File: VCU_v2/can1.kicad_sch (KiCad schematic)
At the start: 6 parts, among them U10 MCP2562FD-E/SN

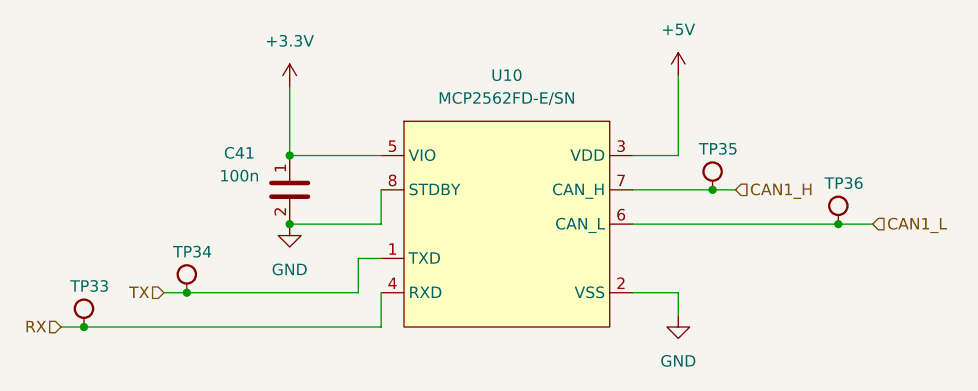
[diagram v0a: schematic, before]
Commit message: placements friggin 80% friggin done shoutout epstein
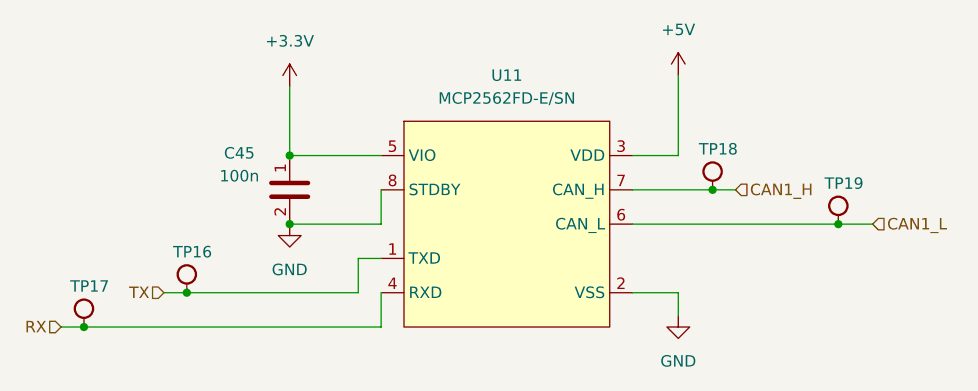
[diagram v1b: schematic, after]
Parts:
- renumbered C41 to C45, TP34 to TP16, TP33 to TP17, TP35 to TP18, TP36 to TP19, U10 to U11
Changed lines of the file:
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@@
 		(dnp no)
 		(fields_autoplaced yes)
-		(property "Reference" "#PWR055"
+		(property "Reference" "#PWR075"
 			(at 114.3 66.04 0)
 			(effects
@@
 			(project ""
 				(path "/4ee6c2ad-9a1b-4276-b3cf-1cc8dc52967e/9e80ce31-2e03-4996-9ce1-7444f7c213d1/6a8587bb-cd3f-4184-88f1-dc60fd50b84f"
-					(reference "#PWR055")
+					(reference "#PWR075")
 					(unit 1)
 				)
@@
 		(on_board yes)
 		(dnp no)
-		(property "Reference" "TP36"
+		(property "Reference" "TP19"
 			(at 173.7368 72.2137 0)
 			(effects
@@
 			(project "VCU_v1"
 				(path "/4ee6c2ad-9a1b-4276-b3cf-1cc8dc52967e/9e80ce31-2e03-4996-9ce1-7444f7c213d1/6a8587bb-cd3f-4184-88f1-dc60fd50b84f"
-					(reference "TP36")
+					(reference "TP19")
 					(unit 1)
 				)
@@
 		(dnp no)
 		(fields_autoplaced yes)
-		(property "Reference" "#PWR057"
+		(property "Reference" "#PWR076"
 			(at 157.48 64.77 0)
 			(effects
@@
 			(project ""
 				(path "/4ee6c2ad-9a1b-4276-b3cf-1cc8dc52967e/9e80ce31-2e03-4996-9ce1-7444f7c213d1/6a8587bb-cd3f-4184-88f1-dc60fd50b84f"
-					(reference "#PWR057")
+					(reference "#PWR076")
 					(unit 1)
 				)
@@
 		(on_board yes)
 		(dnp no)
-		(property "Reference" "TP34"
+		(property "Reference" "TP16"
 			(at 101.3468 79.8337 0)
 			(effects
@@
 			(project "VCU_v1"
 				(path "/4ee6c2ad-9a1b-4276-b3cf-1cc8dc52967e/9e80ce31-2e03-4996-9ce1-7444f7c213d1/6a8587bb-cd3f-4184-88f1-dc60fd50b84f"
-					(reference "TP34")
+					(reference "TP16")
 					(unit 1)
 				)
@@
 		(on_board yes)
 		(dnp no)
-		(property "Reference" "TP35"
+		(property "Reference" "TP18"
 			(at 159.7668 68.4037 0)
 			(effects
@@
 			(project "VCU_v1"
 				(path "/4ee6c2ad-9a1b-4276-b3cf-1cc8dc52967e/9e80ce31-2e03-4996-9ce1-7444f7c213d1/6a8587bb-cd3f-4184-88f1-dc60fd50b84f"
-					(reference "TP35")
+					(reference "TP18")
 					(unit 1)
 				)
@@
 		(on_board yes)
 		(dnp no)
-		(property "Reference" "TP33"
+		(property "Reference" "TP17"
 			(at 89.9168 83.6437 0)
 			(effects
@@
 			(project "VCU_v1"
 				(path "/4ee6c2ad-9a1b-4276-b3cf-1cc8dc52967e/9e80ce31-2e03-4996-9ce1-7444f7c213d1/6a8587bb-cd3f-4184-88f1-dc60fd50b84f"
-					(reference "TP33")
+					(reference "TP17")
 					(unit 1)
 				)
@@
 		(on_board yes)
 		(dnp no)
-		(property "Reference" "U10"
+		(property "Reference" "U11"
 			(at 138.43 60.96 0)
 			(effects
@@
 			(project ""
 				(path "/4ee6c2ad-9a1b-4276-b3cf-1cc8dc52967e/9e80ce31-2e03-4996-9ce1-7444f7c213d1/6a8587bb-cd3f-4184-88f1-dc60fd50b84f"
-					(reference "U10")
+					(reference "U11")
 					(unit 1)
 				)
@@
 		(dnp no)
 		(fields_autoplaced yes)
-		(property "Reference" "#PWR058"
+		(property "Reference" "#PWR077"
 			(at 157.48 93.98 0)
 			(effects
@@
 			(project ""
 				(path "/4ee6c2ad-9a1b-4276-b3cf-1cc8dc52967e/9e80ce31-2e03-4996-9ce1-7444f7c213d1/6a8587bb-cd3f-4184-88f1-dc60fd50b84f"
-					(reference "#PWR058")
+					(reference "#PWR077")
 					(unit 1)
 				)
@@
 		(on_board yes)
 		(dnp no)
-		(property "Reference" "C41"
+		(property "Reference" "C45"
 			(at 108.712 69.596 0)
 			(effects
@@
 			(project ""
 				(path "/4ee6c2ad-9a1b-4276-b3cf-1cc8dc52967e/9e80ce31-2e03-4996-9ce1-7444f7c213d1/6a8587bb-cd3f-4184-88f1-dc60fd50b84f"
-					(reference "C41")
+					(reference "C45")
 					(unit 1)
 				)
@@
 		(dnp no)
 		(fields_autoplaced yes)
-		(property "Reference" "#PWR056"
+		(property "Reference" "#PWR012"
 			(at 114.3 83.82 0)
 			(effects
@@
 			(project ""
 				(path "/4ee6c2ad-9a1b-4276-b3cf-1cc8dc52967e/9e80ce31-2e03-4996-9ce1-7444f7c213d1/6a8587bb-cd3f-4184-88f1-dc60fd50b84f"
-					(reference "#PWR056")
+					(reference "#PWR012")
 					(unit 1)
 				)

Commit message: vcu v2 schematics done
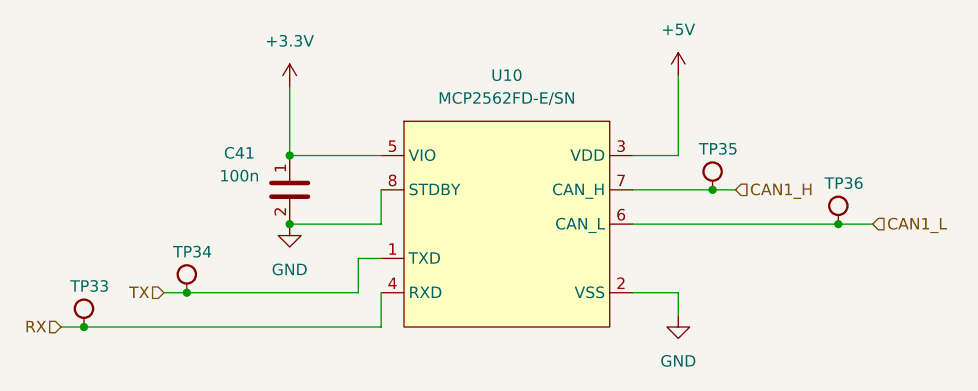
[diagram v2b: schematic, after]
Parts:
- renumbered C45 to C41, TP17 to TP33, TP16 to TP34, TP18 to TP35, TP19 to TP36, U11 to U10
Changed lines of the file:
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@@
 		(dnp no)
 		(fields_autoplaced yes)
-		(property "Reference" "#PWR075"
+		(property "Reference" "#PWR055"
 			(at 114.3 66.04 0)
 			(effects
@@
 			(project ""
 				(path "/4ee6c2ad-9a1b-4276-b3cf-1cc8dc52967e/9e80ce31-2e03-4996-9ce1-7444f7c213d1/6a8587bb-cd3f-4184-88f1-dc60fd50b84f"
-					(reference "#PWR075")
+					(reference "#PWR055")
 					(unit 1)
 				)
@@
 		(on_board yes)
 		(dnp no)
-		(property "Reference" "TP19"
+		(property "Reference" "TP36"
 			(at 173.7368 72.2137 0)
 			(effects
@@
 			(project "VCU_v1"
 				(path "/4ee6c2ad-9a1b-4276-b3cf-1cc8dc52967e/9e80ce31-2e03-4996-9ce1-7444f7c213d1/6a8587bb-cd3f-4184-88f1-dc60fd50b84f"
-					(reference "TP19")
+					(reference "TP36")
 					(unit 1)
 				)
@@
 		(dnp no)
 		(fields_autoplaced yes)
-		(property "Reference" "#PWR076"
+		(property "Reference" "#PWR057"
 			(at 157.48 64.77 0)
 			(effects
@@
 			(project ""
 				(path "/4ee6c2ad-9a1b-4276-b3cf-1cc8dc52967e/9e80ce31-2e03-4996-9ce1-7444f7c213d1/6a8587bb-cd3f-4184-88f1-dc60fd50b84f"
-					(reference "#PWR076")
+					(reference "#PWR057")
 					(unit 1)
 				)
@@
 		(on_board yes)
 		(dnp no)
-		(property "Reference" "TP16"
+		(property "Reference" "TP34"
 			(at 101.3468 79.8337 0)
 			(effects
@@
 			(project "VCU_v1"
 				(path "/4ee6c2ad-9a1b-4276-b3cf-1cc8dc52967e/9e80ce31-2e03-4996-9ce1-7444f7c213d1/6a8587bb-cd3f-4184-88f1-dc60fd50b84f"
-					(reference "TP16")
+					(reference "TP34")
 					(unit 1)
 				)
@@
 		(on_board yes)
 		(dnp no)
-		(property "Reference" "TP18"
+		(property "Reference" "TP35"
 			(at 159.7668 68.4037 0)
 			(effects
@@
 			(project "VCU_v1"
 				(path "/4ee6c2ad-9a1b-4276-b3cf-1cc8dc52967e/9e80ce31-2e03-4996-9ce1-7444f7c213d1/6a8587bb-cd3f-4184-88f1-dc60fd50b84f"
-					(reference "TP18")
+					(reference "TP35")
 					(unit 1)
 				)
@@
 		(on_board yes)
 		(dnp no)
-		(property "Reference" "TP17"
+		(property "Reference" "TP33"
 			(at 89.9168 83.6437 0)
 			(effects
@@
 			(project "VCU_v1"
 				(path "/4ee6c2ad-9a1b-4276-b3cf-1cc8dc52967e/9e80ce31-2e03-4996-9ce1-7444f7c213d1/6a8587bb-cd3f-4184-88f1-dc60fd50b84f"
-					(reference "TP17")
+					(reference "TP33")
 					(unit 1)
 				)
@@
 		(on_board yes)
 		(dnp no)
-		(property "Reference" "U11"
+		(property "Reference" "U10"
 			(at 138.43 60.96 0)
 			(effects
@@
 			(project ""
 				(path "/4ee6c2ad-9a1b-4276-b3cf-1cc8dc52967e/9e80ce31-2e03-4996-9ce1-7444f7c213d1/6a8587bb-cd3f-4184-88f1-dc60fd50b84f"
-					(reference "U11")
+					(reference "U10")
 					(unit 1)
 				)
@@
 		(dnp no)
 		(fields_autoplaced yes)
-		(property "Reference" "#PWR077"
+		(property "Reference" "#PWR058"
 			(at 157.48 93.98 0)
 			(effects
@@
 			(project ""
 				(path "/4ee6c2ad-9a1b-4276-b3cf-1cc8dc52967e/9e80ce31-2e03-4996-9ce1-7444f7c213d1/6a8587bb-cd3f-4184-88f1-dc60fd50b84f"
-					(reference "#PWR077")
+					(reference "#PWR058")
 					(unit 1)
 				)
@@
 		(on_board yes)
 		(dnp no)
-		(property "Reference" "C45"
+		(property "Reference" "C41"
 			(at 108.712 69.596 0)
 			(effects
@@
 			(project ""
 				(path "/4ee6c2ad-9a1b-4276-b3cf-1cc8dc52967e/9e80ce31-2e03-4996-9ce1-7444f7c213d1/6a8587bb-cd3f-4184-88f1-dc60fd50b84f"
-					(reference "C45")
+					(reference "C41")
 					(unit 1)
 				)
@@
 		(dnp no)
 		(fields_autoplaced yes)
-		(property "Reference" "#PWR012"
+		(property "Reference" "#PWR056"
 			(at 114.3 83.82 0)
 			(effects
@@
 			(project ""
 				(path "/4ee6c2ad-9a1b-4276-b3cf-1cc8dc52967e/9e80ce31-2e03-4996-9ce1-7444f7c213d1/6a8587bb-cd3f-4184-88f1-dc60fd50b84f"
-					(reference "#PWR012")
+					(reference "#PWR056")
 					(unit 1)
 				)
